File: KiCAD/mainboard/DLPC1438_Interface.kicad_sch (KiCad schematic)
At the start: 94 parts, among them J10 Conn_01x05_Pin, J2 Conn_01x07_Pin, J29 Conn_01x04_Pin, J3 Conn_02x05_Odd_Even, J31 Conn_01x08_Pin, J4 Conn_01x05_Pin, U12 ECS-2520MV-xxx-xx, U13 MX25L3233FM2, U14 SN74AUP1G06DCKR, U16 DLPC1438ZEZ, U22 TXS0102DCU, U37 TXS0102DCU, U5 SN74AUP1G06DCKR, U7 SN74AUP1G06DCKR

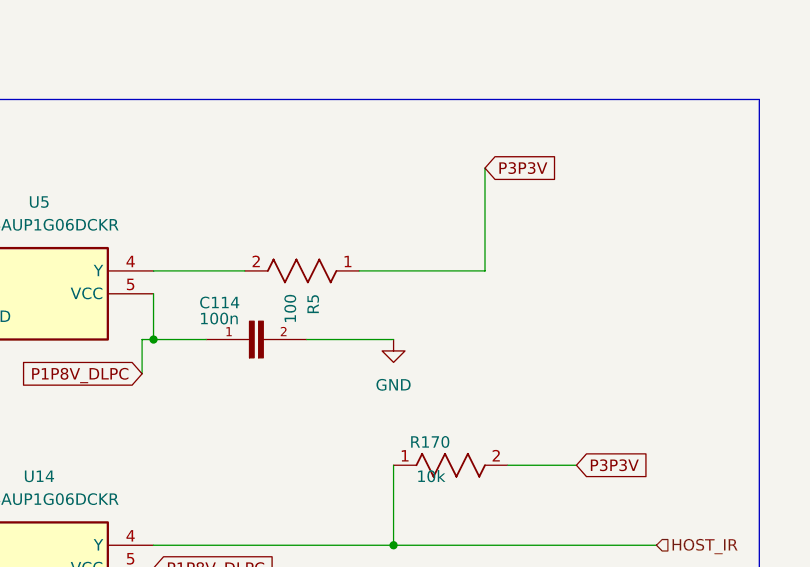
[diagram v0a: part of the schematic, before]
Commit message: more layout stuff
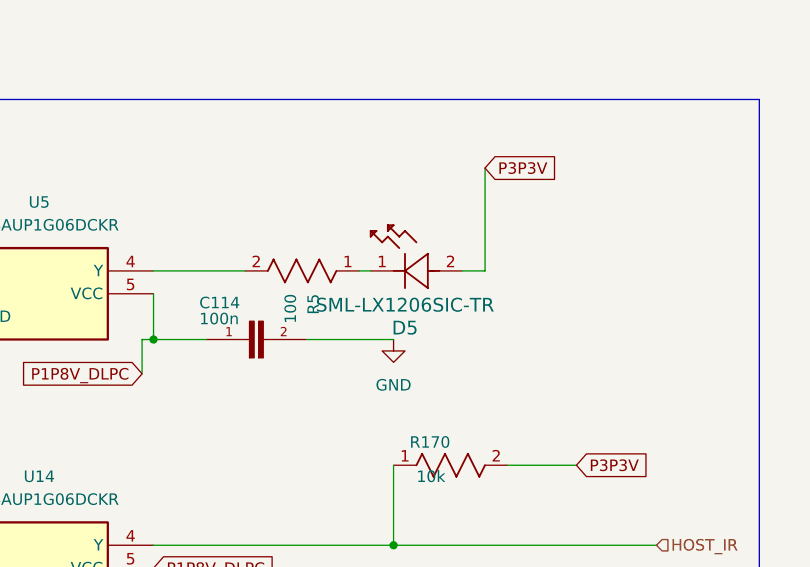
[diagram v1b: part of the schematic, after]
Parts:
- added D5: SML-LX1206SIC-TR, tp_library:LED_SML-LX1206SIC-TR_LUM-M, symbol ul_SML-LX1206SIC-TR:SML-LX1206SIC-TR
- C108, C112, C114, C115, C120, C121, C125, C126, C127, C128, C129, C130, C131, C132, C133, C134, C138, C139, C140, C141, C142, C143, C144, C145, C155, C156, C157, C170, C171, C238, C239, C7: footprint CAPC2012X70 -> tp_library:CAP_CL05_SAM
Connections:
- net P3P3V: now also D5.2; no longer R5.1
- new net: D5.1, R5.1
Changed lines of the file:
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@@
 	(wire
 		(pts
-			(xy 125.73 220.98) (xy 139.7 220.98)
+			(xy 125.73 220.98) (xy 127 220.98)
 		)
 		(stroke
@@
 	(wire
 		(pts
+			(xy 137.16 220.98) (xy 139.7 220.98)
+		)
+		(stroke
+			(width 0)
+			(type default)
+		)
+	)
+	(wire
+		(pts
 			(xy 417.83 102.87) (xy 431.8 102.87)
 		)
@@
 			)
 		)
-		(property "Footprint" "CAPC2012X70"
+		(property "Footprint" "tp_library:CAP_CL05_SAM"
 			(at 513.08 226.06 0)
 			(effects
@@
 	)
 	(symbol
+		(lib_id "ul_SML-LX1206SIC-TR:SML-LX1206SIC-TR")
+		(at 137.16 220.98 0)
+		(mirror y)
+		(unit 1)
+		(exclude_from_sim no)
+		(in_bom yes)
+		(on_board yes)
+		(dnp no)
+		(property "Reference" "D5"
+			(at 130.81 227.33 0)
+			(effects
+				(font
+					(size 1.524 1.524)
+				)
+			)
+		)
+		(property "Value" "SML-LX1206SIC-TR"
+			(at 130.81 224.79 0)
+			(effects
+				(font
+					(size 1.524 1.524)
+				)
+			)
+		)
+		(property "Footprint" "tp_library:LED_SML-LX1206SIC-TR_LUM-M"
+			(at 137.16 220.98 0)
+			(effects
+				(font
+					(size 1.27 1.27)
+					(italic yes)
+				)
+				(hide yes)
+			)
+		)
+		(property "Datasheet" "SML-LX1206SIC-TR"
+			(at 137.16 220.98 0)
+			(effects
+				(font
+					(size 1.27 1.27)
+					(italic yes)
+				)
+				(hide yes)
+			)
+		)
+		(property "Description" ""
+			(at 137.16 220.98 0)
+			(effects
+				(font
+					(size 1.27 1.27)
+				)
+				(hide yes)
+			)
+		)
+		(pin "2"
+		)
+		(pin "1"
+		)
+		(instances
+			(project "mainboard"
+				(path "/38e83f42-2cf9-4799-a46f-ca415d95b90a/a69a407c-1a7c-4ac9-a9eb-cd67809c5ec0"
+					(reference "D5")
+					(unit 1)
+				)
+			)
+		)
+	)
+	(symbol
 		(lib_id "ERJP06F3301V:ERJP06F3301V")
 		(at 64.77 297.18 90)
@@
 			)
 		)
-		(property "Footprint" "CAPC2012X70"
+		(property "Footprint" "tp_library:CAP_CL05_SAM"
 			(at 251.46 58.42 0)
 			(effects
@@
 			)
 		)
-		(property "Footprint" "CAPC2012X70"
+		(property "Footprint" "tp_library:CAP_CL05_SAM"
 			(at 114.3 228.6 0)
 			(effects
@@
 			)
 		)
-		(property "Footprint" "CAPC2012X70"
+		(property "Footprint" "tp_library:CAP_CL05_SAM"
 			(at 186.69 58.42 0)
 			(effects
@@
 			)
 		)
-		(property "Footprint" "CAPC2012X70"
+		(property "Footprint" "tp_library:CAP_CL05_SAM"
 			(at 260.35 58.42 0)
 			(effects
@@
 			)
 		)
-		(property "Footprint" "CAPC2012X70"
+		(property "Footprint" "tp_library:CAP_CL05_SAM"
 			(at 123.19 133.35 0)
 			(effects
@@
 			)
 		)
-		(property "Footprint" "CAPC2012X70"
+		(property "Footprint" "tp_library:CAP_CL05_SAM"
 			(at 252.73 134.62 0)
 			(effects
@@
 			)
 		)
-		(property "Footprint" "CAPC2012X70"
+		(property "Footprint" "tp_library:CAP_CL05_SAM"
 			(at 58.42 58.42 0)
 			(effects
@@
 			)
 		)
-		(property "Footprint" "CAPC2012X70"
+		(property "Footprint" "tp_library:CAP_CL05_SAM"
 			(at 318.77 132.08 0)
 			(effects
@@
 			)
 		)
-		(property "Footprint" "CAPC2012X70"
+		(property "Footprint" "tp_library:CAP_CL05_SAM"
 			(at 270.51 58.42 0)
 			(effects
@@
 			)
 		)
-		(property "Footprint" "CAPC2012X70"
+		(property "Footprint" "tp_library:CAP_CL05_SAM"
 			(at 242.57 224.79 0)
 			(effects
@@
 			)
 		)
-		(property "Footprint" "CAPC2012X70"
+		(property "Footprint" "tp_library:CAP_CL05_SAM"
 			(at 483.87 180.34 0)
 			(effects
@@
 			)
 		)
-		(property "Footprint" "CAPC2012X70"
+		(property "Footprint" "tp_library:CAP_CL05_SAM"
 			(at 120.65 59.69 0)
 			(effects
@@
 			)
 		)
-		(property "Footprint" "CAPC2012X70"
+		(property "Footprint" "tp_library:CAP_CL05_SAM"
 			(at 72.39 57.15 0)
 			(effects
@@
 			)
 		)
-		(property "Footprint" "CAPC2012X70"
+		(property "Footprint" "tp_library:CAP_CL05_SAM"
 			(at 219.71 58.42 0)
 			(effects
@@
 			)
 		)
-		(property "Footprint" "CAPC2012X70"
+		(property "Footprint" "tp_library:CAP_CL05_SAM"
 			(at 135.89 59.69 0)
 			(effects
@@
 			)
 		)
-		(property "Footprint" "CAPC2012X70"
+		(property "Footprint" "tp_library:CAP_CL05_SAM"
 			(at 210.82 58.42 0)
 			(effects
@@
 			)
 		)
-		(property "Footprint" "CAPC2012X70"
+		(property "Footprint" "tp_library:CAP_CL05_SAM"
 			(at 201.93 58.42 0)
 			(effects
@@
 			)
 		)
-		(property "Footprint" "CAPC2012X70"
+		(property "Footprint" "tp_library:CAP_CL05_SAM"
 			(at 194.31 58.42 0)
 			(effects
@@
 			)
 		)
-		(property "Footprint" "CAPC2012X70"
+		(property "Footprint" "tp_library:CAP_CL05_SAM"
 			(at 66.04 57.15 0)
 			(effects
@@
 			)
 		)
-		(property "Footprint" "CAPC2012X70"
+		(property "Footprint" "tp_library:CAP_CL05_SAM"
 			(at 242.57 134.62 0)
 			(effects
@@
 			)
 		)
-		(property "Footprint" "CAPC2012X70"
+		(property "Footprint" "tp_library:CAP_CL05_SAM"
 			(at 146.05 309.88 0)
 			(effects
@@
 			)
 		)
-		(property "Footprint" "CAPC2012X70"
+		(property "Footprint" "tp_library:CAP_CL05_SAM"
 			(at 95.25 309.88 0)
 			(effects
@@
 			)
 		)
-		(property "Footprint" "CAPC2012X70"
+		(property "Footprint" "tp_library:CAP_CL05_SAM"
 			(at 549.91 139.7 0)
 			(effects
@@
 			)
 		)
-		(property "Footprint" "CAPC2012X70"
+		(property "Footprint" "tp_library:CAP_CL05_SAM"
 			(at 245.11 58.42 0)
 			(effects
@@
 			)
 		)
-		(property "Footprint" "CAPC2012X70"
+		(property "Footprint" "tp_library:CAP_CL05_SAM"
 			(at 142.24 59.69 0)
 			(effects
@@
 			)
 		)
-		(property "Footprint" "CAPC2012X70"
+		(property "Footprint" "tp_library:CAP_CL05_SAM"
 			(at 307.34 181.61 0)
 			(effects
@@
 			)
 		)
-		(property "Footprint" "CAPC2012X70"
+		(property "Footprint" "tp_library:CAP_CL05_SAM"
 			(at 236.22 58.42 0)
 			(effects
@@
 			)
 		)
-		(property "Footprint" "CAPC2012X70"
+		(property "Footprint" "tp_library:CAP_CL05_SAM"
 			(at 227.33 58.42 0)
 			(effects
@@
 			)
 		)
-		(property "Footprint" "CAPC2012X70"
+		(property "Footprint" "tp_library:CAP_CL05_SAM"
 			(at 563.88 147.32 0)
 			(effects
@@
 			)
 		)
-		(property "Footprint" "CAPC2012X70"
+		(property "Footprint" "tp_library:CAP_CL05_SAM"
 			(at 80.01 57.15 0)
 			(effects
@@
 			)
 		)
-		(property "Footprint" "CAPC2012X70"
+		(property "Footprint" "tp_library:CAP_CL05_SAM"
 			(at 128.27 59.69 0)
 			(effects
